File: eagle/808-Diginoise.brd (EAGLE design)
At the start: 100 x 80 mm, 28 parts, among them IC1 4584N, IC2 TL071P, U1 POWER

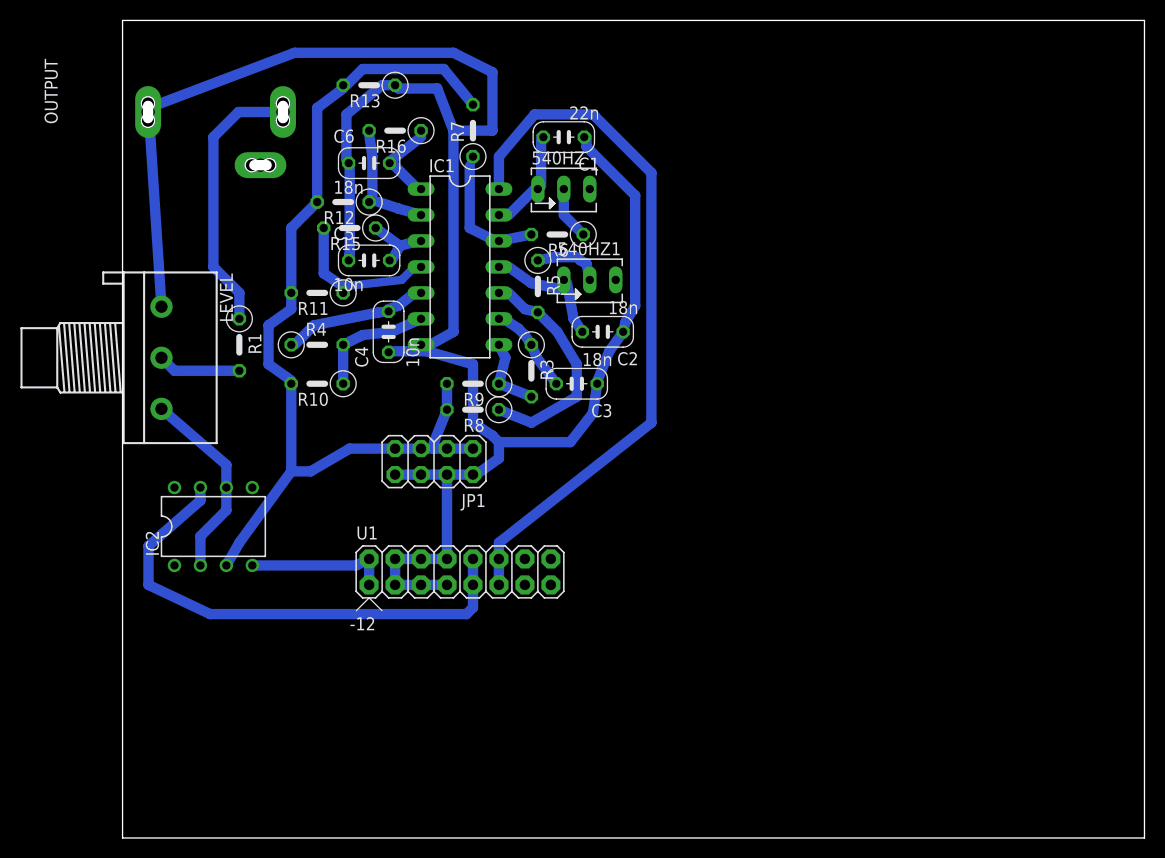
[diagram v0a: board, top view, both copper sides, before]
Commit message: gcode
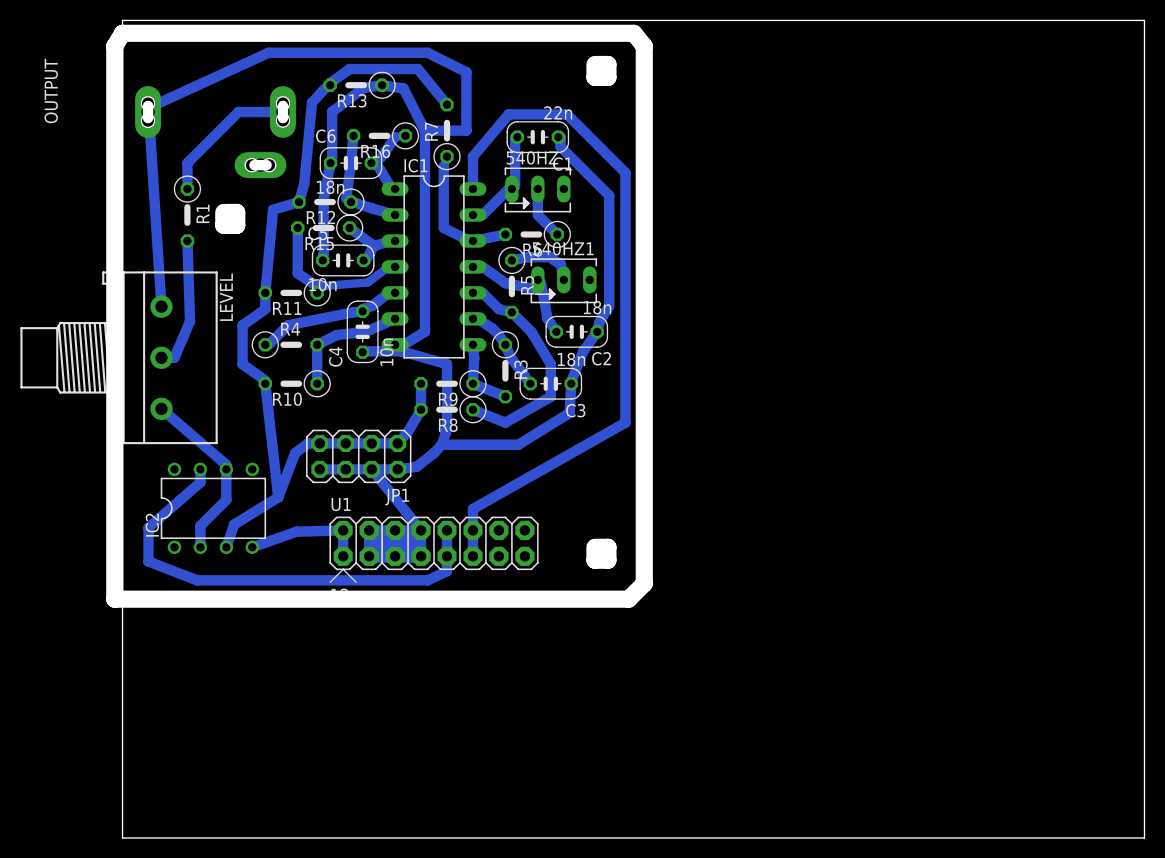
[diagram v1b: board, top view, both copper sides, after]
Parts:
- moved R1 13.7 mm to (6.35, 61.0)
- moved JP1 7.38 mm to (23.1, 37.3)
- moved U1 3.78 mm to (27.9, 28.8)
- moved C3 2.54 mm to (41.9, 44.5)
- moved IC1 2.54 mm to (30.5, 55.9)
- moved R15 2.54 mm to (19.7, 59.7)
- moved 540HZ 2.54 mm to (40.6, 63.5)
- moved 540HZ1 2.54 mm to (43.2, 54.6)
- moved C1 2.54 mm to (40.6, 68.6)
- moved C2 2.54 mm to (44.5, 49.5)
- moved C4 2.54 mm to (23.5, 49.5)
- moved C5 2.54 mm to (21.6, 56.5)
- moved R10 2.54 mm to (16.5, 44.5)
- moved R11 2.54 mm to (16.5, 53.3)
- moved R3 2.54 mm to (37.5, 45.7)
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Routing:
- net N$16: track 26.7 -> 14.0 mm
- net N$18: track 93.6 -> 88.2 mm
- net N$7: track 8.15 -> 13.3 mm
- net +12V: track 49.2 -> 45.1 mm
- net -12V: track 14.1 -> 11.7 mm
- net GND: track 208.9 -> 206.4 mm
- net N$2: track 19.3 -> 17.5 mm
- net +5V: track 69.9 -> 68.6 mm
- net N$11: track 12.4 -> 11.6 mm
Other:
- board size 100 x 80 mm -> 100.8 x 80 mm
